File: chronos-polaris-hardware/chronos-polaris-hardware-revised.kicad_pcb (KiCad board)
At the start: 2 copper layers, 40 x 50 mm, 102 parts, among them J1 Conn_01x03_Pin, J2 Conn_01x03_Pin, J3 Conn_01x03_Pin, J4 Conn_01x03_Pin, J5 Conn_01x03_Pin, J6 Conn_01x04, J7 Conn_01x04, J8 Conn_01x02, J9 691417320006S, P1 WJ124-3_81-6P, Q1 US6K4TR, U1 TLV62130RGTR, U1 TPS62172DSGR, U10 MSK12C02-HB, U11 TPS62172DSGR, U12 AP20P30Q, U14 FC-B1010RGBT-HG, U15 TYPE-C_14PLC-H10_0, U2 ESP32-S2-SOLO-2-N4, U3 BMI088, U4 BMP280, U4 TYPE-C_14PLC-H10_0, U5 TF_PUSH, U6 TLV62130RGTR, U6 TPS629206DRLR, U7 AP20P30Q, U8 2N7002KDW_72K, U9 BMP280

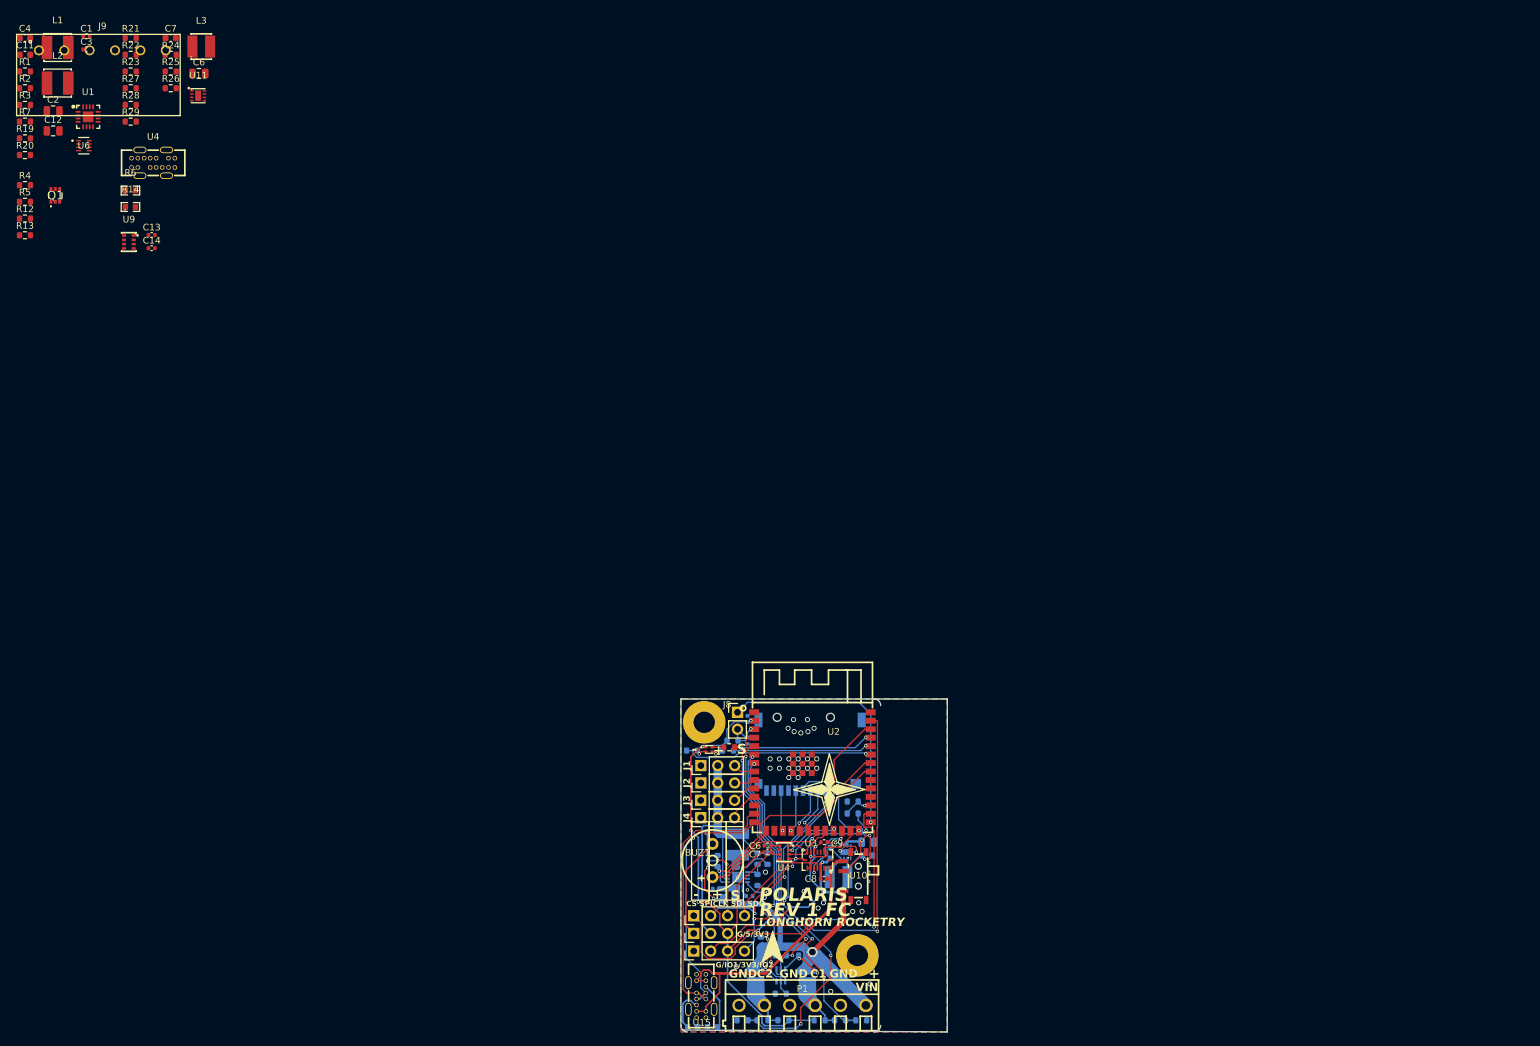
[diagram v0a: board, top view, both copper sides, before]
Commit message: fix merge conflicts . - Rishik B.
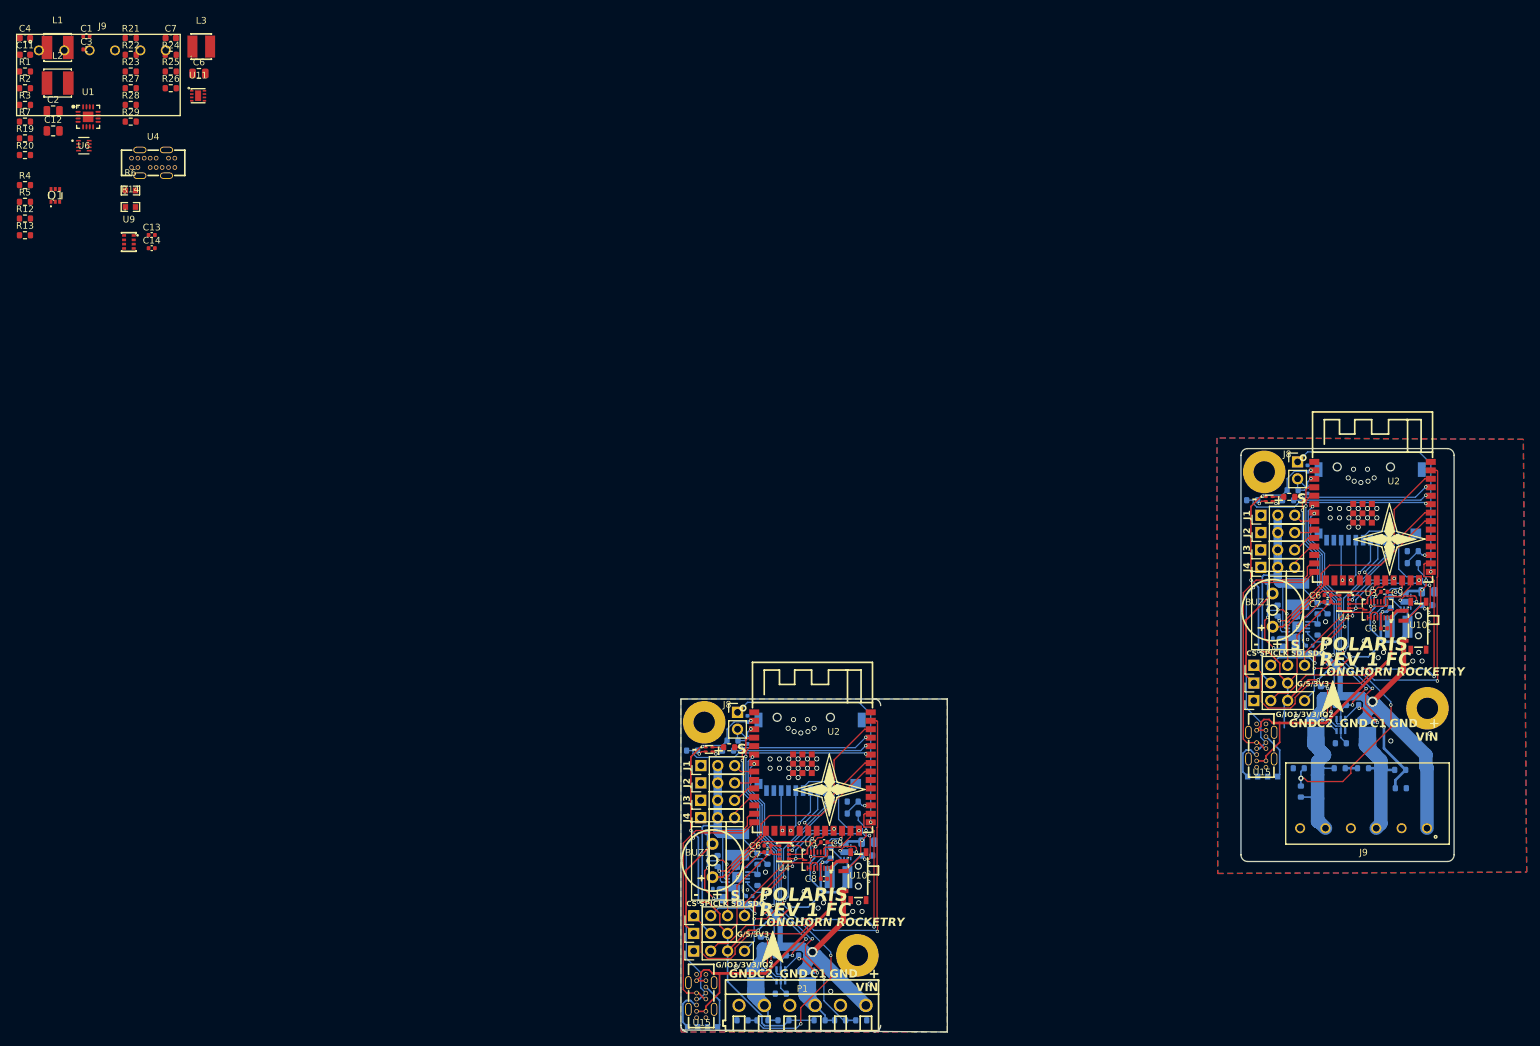
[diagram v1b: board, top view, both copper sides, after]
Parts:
- added BUZ1: HNB09A03, polaris-fp:BUZ-TH_BD9.0-P5.00-D0.6-FD, F.Cu at (188.8, 86.7)
- added C1: 22uF, Capacitor_SMD:C_0603_1608Metric, B.Cu at (212.1, 85.9)
- added C10: 100nF, Capacitor_SMD:C_0402_1005Metric, B.Cu at (194.1, 65.4)
- added C11: 3.3nF, Capacitor_SMD:C_0402_1005Metric, B.Cu at (194.4, 92.0)
- added C12: 100nF, Capacitor_SMD:C_0402_1005Metric, B.Cu at (189.4, 90.9)
- added C2: 10uF, Capacitor_SMD:C_0805_2012Metric, B.Cu at (212.2, 83.9)
- added C3: 22uF, Capacitor_SMD:C_0603_1608Metric, B.Cu at (188.8, 82.4)
- added C4: 10uF, Capacitor_SMD:C_0805_2012Metric, B.Cu at (191.4, 92.4)
- added C5: 100nF, Capacitor_SMD:C_0402_1005Metric, B.Cu at (194.1, 68.7)
- added C6: 100nF, Capacitor_SMD:C_0402_1005Metric, F.Cu at (197.1, 84.4)
- added C7: 100nF, Capacitor_SMD:C_0402_1005Metric, F.Cu at (197.1, 85.4)
- added C8: 100nF, Capacitor_SMD:C_0402_1005Metric, F.Cu at (205.6, 89.4)
- added C9: 100nF, Capacitor_SMD:C_0402_1005Metric, F.Cu at (205.6, 83.9)
- added H1: MountingHole, MountingHole:MountingHole_3.2mm_M3_Pad, F.Cu at (212.1, 101.4)
- added H4: MountingHole, MountingHole:MountingHole_3.2mm_M3_Pad, F.Cu at (187.6, 65.9)
- added J1: Conn_01x03_Pin, Connector_PinHeader_2.54mm:PinHeader_1x03_P2.54mm_Vertical, F.Cu at (187.1, 72.4)
- added J2: Conn_01x03_Pin, Connector_PinHeader_2.54mm:PinHeader_1x03_P2.54mm_Vertical, F.Cu at (187.1, 75.0)
- added J3: Conn_01x03_Pin, Connector_PinHeader_2.54mm:PinHeader_1x03_P2.54mm_Vertical, F.Cu at (187.1, 77.6)
- added J4: Conn_01x03_Pin, Connector_PinHeader_2.54mm:PinHeader_1x03_P2.54mm_Vertical, F.Cu at (187.1, 80.2)
- added J5: Conn_01x03_Pin, Connector_PinHeader_2.54mm:PinHeader_1x03_P2.54mm_Vertical, F.Cu at (186.0, 97.6)
- added J6: Conn_01x04, Connector_PinHeader_2.54mm:PinHeader_1x04_P2.54mm_Vertical, F.Cu at (186.0, 100.2)
- added J7: Conn_01x04, Connector_PinHeader_2.54mm:PinHeader_1x04_P2.54mm_Vertical, F.Cu at (186.0, 94.9)
- added J8: Conn_01x02, Connector_PinHeader_2.54mm:PinHeader_1x02_P2.54mm_Vertical, F.Cu at (192.6, 64.4)
- added J9: 691417320006S, polaris-fp:691417320006S, F.Cu at (202.5, 119.4)
- added L1: 2.2uH, polaris-fp:IND-SMD_L3.0-W3.0, B.Cu at (207.8, 89.2)
- added L2: 2.2uH, polaris-fp:IND-SMD_L4.0-W4.0, B.Cu at (192.6, 84.2)
- added R1: 100k, Resistor_SMD:R_0603_1608Metric, B.Cu at (206.6, 85.5)
- added R10: 51, Resistor_SMD:R_0603_1608Metric, B.Cu at (191.2, 70.2)
- added R11: 100, Resistor_SMD:R_0603_1608Metric, F.Cu at (191.3, 69.7)
- added R12: 0603WAF5101T5E, polaris-fp:R0603, B.Cu at (185.9, 111.7)
- added R13: 0603WAF5101T5E, polaris-fp:R0603, B.Cu at (188.8, 111.7)
- added R14: 30k, Resistor_SMD:R_0603_1608Metric, B.Cu at (208.0, 110.7)
- added R15: 10k, Resistor_SMD:R_0603_1608Metric, B.Cu at (208.1, 113.4)
- added R16: 10k, Resistor_SMD:R_0603_1608Metric, B.Cu at (198.9, 110.4)
- added R17: 30k, Resistor_SMD:R_0603_1608Metric, B.Cu at (193.1, 113.9)
- added R18: 10k, Resistor_SMD:R_0603_1608Metric, B.Cu at (192.8, 110.4)
- added R19: 100k, Resistor_SMD:R_0603_1608Metric, B.Cu at (197.1, 86.4)
- added R2: 10k, Resistor_SMD:R_0603_1608Metric, B.Cu at (196.1, 99.0)
- added R20: 160k, Resistor_SMD:R_0603_1608Metric, B.Cu at (195.6, 86.4)
- added R21: 10k, Resistor_SMD:R_0603_1608Metric, B.Cu at (189.6, 86.7)
- added R22: 30k, Resistor_SMD:R_0603_1608Metric, B.Cu at (209.9, 79.6)
- added R23: 10k, Resistor_SMD:R_0603_1608Metric, B.Cu at (209.9, 77.8)
- added R3: 10k, Resistor_SMD:R_0603_1608Metric, B.Cu at (202.6, 100.9)
- added R4: 10k, Resistor_SMD:R_0603_1608Metric, B.Cu at (199.1, 100.9)
- added R5: 10k, Resistor_SMD:R_0603_1608Metric, B.Cu at (199.1, 106.7)
- added R6: 10k, Resistor_SMD:R_0603_1608Metric, B.Cu at (202.4, 110.4)
- added R7: 30k, Resistor_SMD:R_0603_1608Metric, B.Cu at (195.6, 89.6)
- added R8: 10k, Resistor_SMD:R_0603_1608Metric, B.Cu at (191.8, 68.7)
- added R9: 51, Resistor_SMD:R_0603_1608Metric, B.Cu at (185.8, 70.2)
- added U1: TPS62172DSGR, polaris-fp:WSON-8_L2.0-W2.0-P0.50-TL-EP, B.Cu at (208.8, 85.4)
- added U10: MSK12C02-HB, polaris-fp:SW-TH_MSK12C02-HB-1, F.Cu at (210.2, 89.0)
- added U12: AP20P30Q, polaris-fp:DFN-8_L3.3-W3.0-P0.65-LS3.3-BL-EP, B.Cu at (203.1, 104.7)
- added U14: FC-B1010RGBT-HG, polaris-fp:LED-ARRAY-SMD_4P-L1.0-W1.0-TR-RD, F.Cu at (188.3, 70.0)
- added U15: TYPE-C_14PLC-H10_0, polaris-fp:USB-C-TH_SHOUHAN_TYPE-C-14PLC-H10.0, F.Cu at (187.1, 107.0)
- added U2: ESP32-S2-SOLO-2-N4, polaris-fp:WIRELM-SMD_ESP32-S3-WROOM-1, F.Cu at (203.9, 73.3)
- added U3: BMI088, polaris-fp:LGA-16_L4.5-W3.0-P0.50-BL, F.Cu at (204.6, 86.6)
- added U4: BMP280, polaris-fp:LGA-8_L2.5-W2.0-P0.65_AMP6127, F.Cu at (199.6, 85.4)
- added U5: TF_PUSH, polaris-fp:TF-SMD_TF-PUSH, B.Cu at (203.5, 70.9)
- added U6: TLV62130RGTR, polaris-fp:QFN-16_L3.0-W3.0-P0.50-TL-EP, B.Cu at (192.6, 89.2)
- added U7: AP20P30Q, polaris-fp:DFN-8_L3.3-W3.0-P0.65-LS3.3-BL-EP, B.Cu at (195.3, 104.7)
- added U8: 2N7002KDW_72K, polaris-fp:SOT-363_L2.1-W1.3-P0.65-LS2.3-BL, B.Cu at (199.1, 103.9)
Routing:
- net 3.3V: track 153.2 -> 291.2 mm, vias 11 -> 22
- net /BAT+: track 68.8 -> 148.7 mm, vias 1 -> 2
- net Net-(J6-Pin_2): track 59.9 -> 119.9 mm, vias 2 -> 4
- net /DROGUE DETECT: track 54.7 -> 112.6 mm, vias 3 -> 6
- net Net-(J7-Pin_1): track 57.5 -> 115.0 mm, vias 2 -> 4
- net GND: track 52.7 -> 105.4 mm, vias 46 -> 92
- net /MAIN DETECT: track 48.3 -> 98.5 mm, vias 3 -> 6
- net 5V: track 46.3 -> 92.5 mm
- net /MAIN CTRL: track 45.0 -> 90.1 mm, vias 5 -> 10
- net /USB_5V: track 43.2 -> 86.4 mm
- net Net-(J6-Pin_4): track 42.7 -> 85.5 mm, vias 3 -> 6
- net /DROGUE CTRL: track 39.7 -> 79.4 mm, vias 3 -> 6
- net Net-(U2-IO19): track 38.5 -> 77.0 mm
- net /GPIO0 (BOOTLOADER): track 37.6 -> 75.2 mm, vias 1 -> 2
- net Net-(U2-IO20): track 36.8 -> 73.5 mm, vias 1 -> 2
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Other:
- board size 40 x 50 mm -> 116.1 x 87.6 mm
